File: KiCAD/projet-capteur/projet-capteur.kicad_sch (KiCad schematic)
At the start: 21 parts, among them J1 Power, J2 Analog, J3 Digital/PWM, J4 Digital/PWM, U2 LTC1050

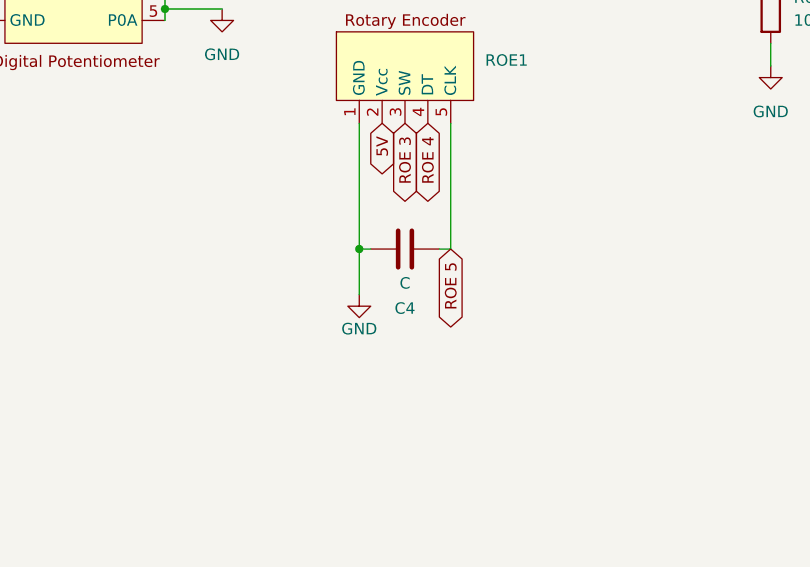
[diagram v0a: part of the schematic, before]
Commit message: Seance Realisation banc de test 17.03
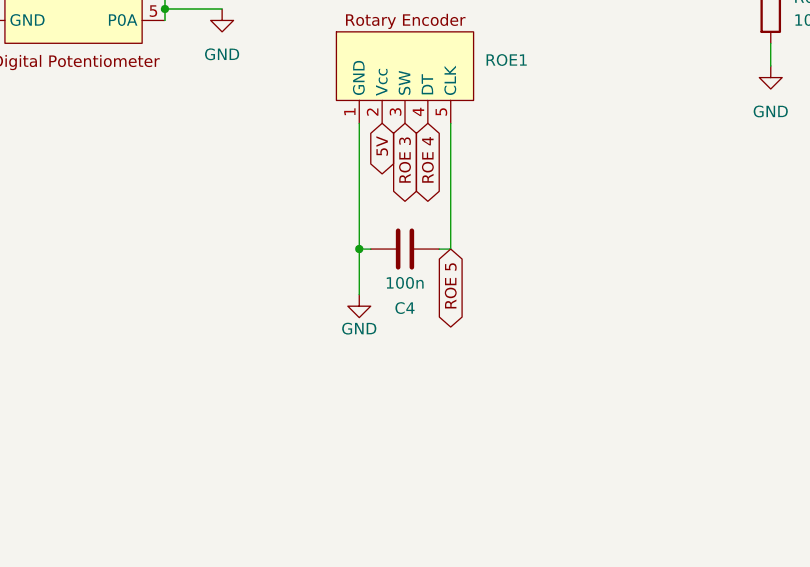
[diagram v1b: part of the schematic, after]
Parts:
- C4: value C -> 100n
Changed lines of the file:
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@@
 			)
 		)
-		(property "Value" "C"
+		(property "Value" "100n"
 			(at 175.26 106.68 90)
 			(effects
